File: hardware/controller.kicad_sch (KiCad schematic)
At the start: 1 part, among them U1 ESP32-C6-WROOM-1

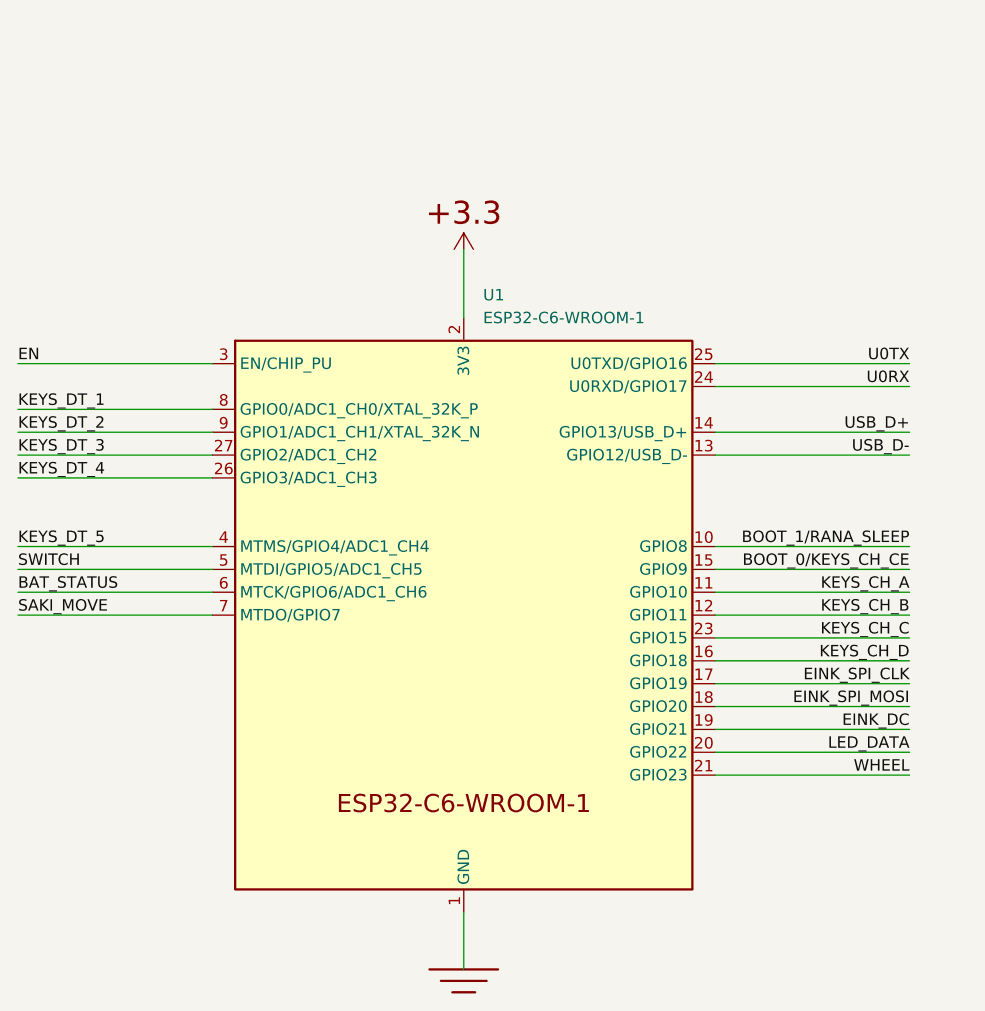
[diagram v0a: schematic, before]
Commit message: :construction: daily update
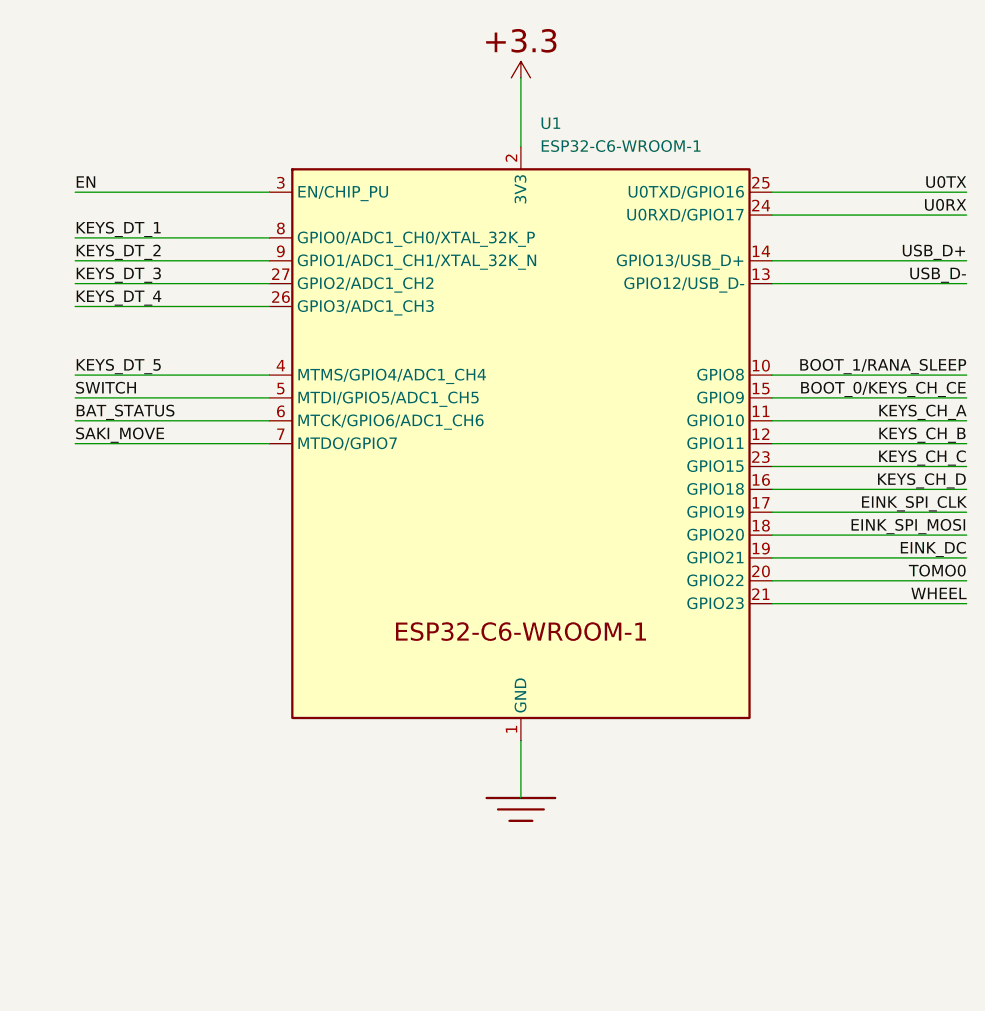
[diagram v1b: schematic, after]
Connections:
- net LED_DATA renamed TOMO0
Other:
- moved on the sheet: U1
